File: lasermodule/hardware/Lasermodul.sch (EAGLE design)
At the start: 78 parts, among them IC1 MEGA8-AI

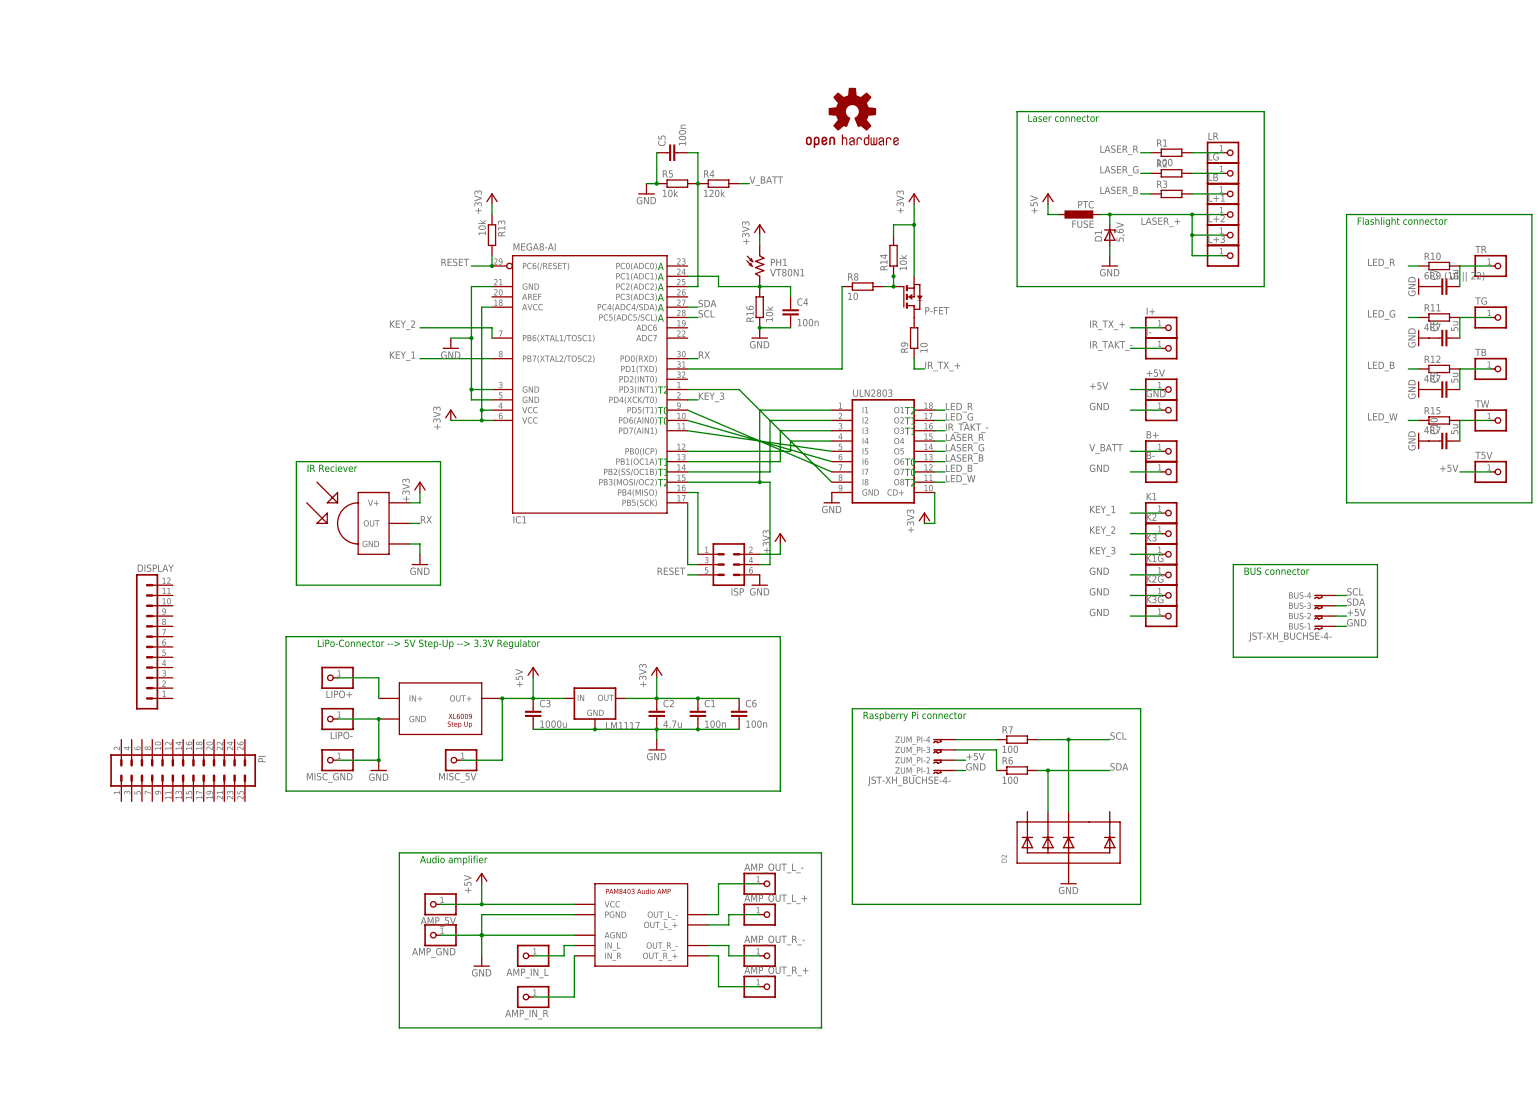
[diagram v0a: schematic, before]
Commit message: weiter gemacht
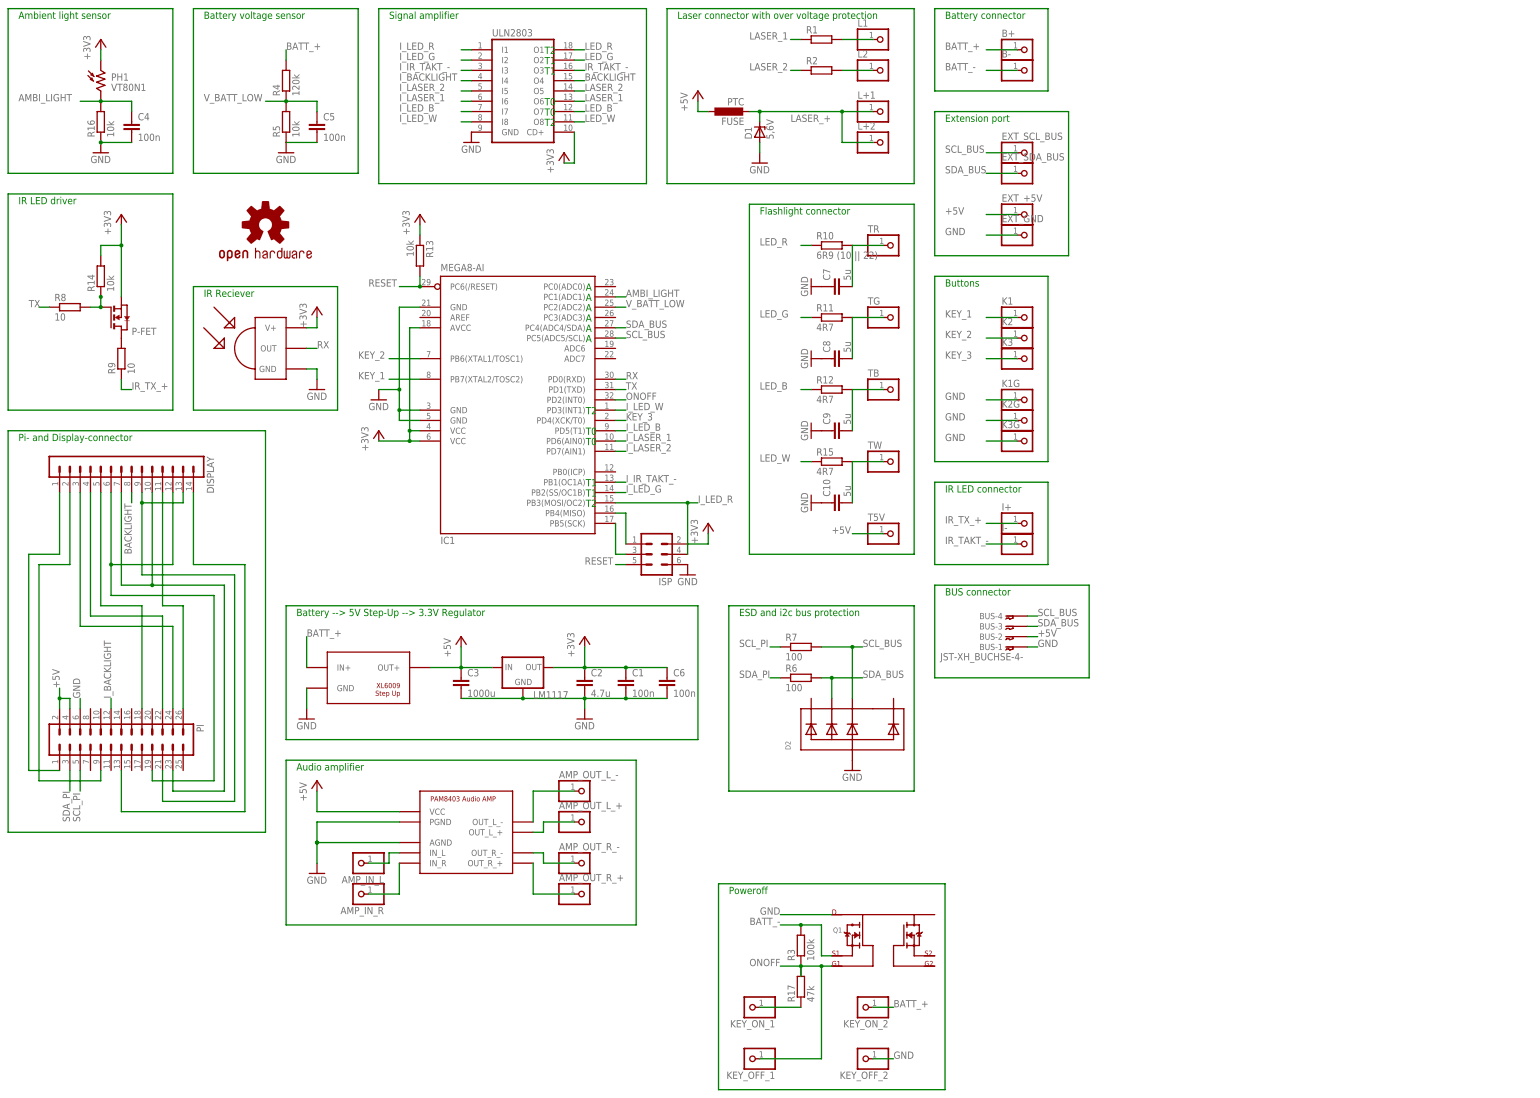
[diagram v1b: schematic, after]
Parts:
- removed +5V, AMP_5V, AMP_GND, GND, L+3, LB, LG, LIPO+, LIPO-, LR, MISC_5V, MISC_GND: (no value), wz:PIN-HEADER-1
- removed ZUM_PI: JST-XH_BUCHSE-4-, wz:JST-XH_BUCHSE-4-
- added EXT_+5V, EXT_GND, EXT_SCL_BUS, EXT_SDA_BUS, KEY_OFF_1, KEY_OFF_2, KEY_ON_1, KEY_ON_2, L1, L2: (no value), wz:PIN-HEADER-1
- added Q1: (no value), wz:CEG8205_DOPPEL_N_FET
- added R17: 47k, wz:R_EU0603
- DISPLAY: device con-lstb:MA12-1 -> wz:PIN-HEADER-DISPLAY
- R1: value 100 -> (none)
- R3: value (none) -> 100k
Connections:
- net LASER_G renamed LASER_2
- net N$1 renamed I_LED_R
- net N$10 renamed I_LED_B
- net N$17 renamed TX
- net N$2 renamed I_LED_G
- net N$26 renamed AMBI_LIGHT
- net N$3 renamed I_IR_TAKT_-
- net N$7 renamed I_LASER_2
- net N$8 renamed I_LED_W
- net N$9 renamed I_LASER_1
- removed net LASER_B: R3.1, ULN2803.O6
- removed net LASER_R: R1.1, ULN2803.O4
- removed net N$14: C5.2, IC1.PC2(ADC2), R4.1, R5.2
- removed net N$19: LB.1, R3.2
- removed net N$27: R7.1, ZUM_PI-4.1
- removed net N$28: R6.1, ZUM_PI-3.1
- removed net N$34: LIPO+.1, U$3.IN+
- removed net N$4: IC1.PB0(ICP), ULN2803.I4
- removed net SCL: BUS-4.1, D2.C3, IC1.PC5(ADC5/SCL), R7.2
- removed net SDA: BUS-3.1, D2.C2, IC1.PC4(ADC4/SDA), R6.2
- removed net V_BATT: B+.1, R4.2
- new net BACKLIGHT: DISPLAY.8, ULN2803.O4
- new net BATT_+: B+.1, KEY_ON_2.1, R4.2, U$3.IN+
- new net BATT_-: B-.1, Q1.S1, R3.2
- new net I_BACKLIGHT: PI.12, ULN2803.I4
- new net LASER_1: R1.1, ULN2803.O6
- new net N$1: DISPLAY.14, PI.13
- new net N$2: DISPLAY.11, PI.26
- new net N$26: KEY_ON_1.1, R17.1
- new net N$44: DISPLAY.1, PI.1
- new net N$45: DISPLAY.2, PI.9
- new net N$47: DISPLAY.5, PI.18
- new net N$48: DISPLAY.12, DISPLAY.6, PI.19
- new net N$49: DISPLAY.13, DISPLAY.9, PI.21
- new net N$50: DISPLAY.4, PI.22
- new net N$51: DISPLAY.10, DISPLAY.7, PI.23
- new net N$52: DISPLAY.3, PI.24
- new net ONOFF: IC1.PD2(INT0), KEY_OFF_1.1, Q1.G1, R17.2, R3.1
- new net SCL_BUS: BUS-4.1, D2.C3, EXT_SCL_BUS.1, IC1.PC5(ADC5/SCL), R7.2
- new net SCL_PI: PI.5, R7.1
- new net SDA_BUS: BUS-3.1, D2.C2, EXT_SDA_BUS.1, IC1.PC4(ADC4/SDA), R6.2
- new net SDA_PI: PI.3, R6.1
- new net V_BATT_LOW: C5.1, IC1.PC2(ADC2), R4.1, R5.2
- net +5V: now also EXT_+5V.1, PI.2, PI.4; no longer +5V.1, AMP_5V.1, MISC_5V.1, ZUM_PI-2.1
- net GND: now also C5.2, EXT_GND.1, KEY_OFF_2.1, PI.6, Q1.D; no longer AMP_GND.1, B-.1, C5.1, GND.1, LIPO-.1, MISC_GND.1, ZUM_PI-1.1
- net LASER_+: no longer L+3.1
- net N$12: now also L1.1; no longer LR.1
- net N$18: now also L2.1; no longer LG.1
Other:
- note added: "Ambient light sensor"
- note added: "Battery --> 5V Step-Up --> 3.3V Regulator"
- note added: "Battery connector"
- note added: "Battery voltage sensor"
- note added: "Buttons"
- note added: "ESD and i2c bus protection"
- note added: "Extension port"
- note added: "IR LED connector"
- note added: "IR LED driver"
- note added: "Laser connector with over voltage protection"
- note added: "Pi- and Display-connector"
- note added: "Poweroff"
- note added: "Signal amplifier"
- note removed: "Laser connector"
- note removed: "LiPo-Connector --> 5V Step-Up --> 3.3V Regulator"
- note removed: "Raspberry Pi connector"
- moved on the sheet: AMP_IN_L, AMP_IN_R, AMP_OUT_L_+, AMP_OUT_L_-, AMP_OUT_R_+, AMP_OUT_R_-, B+, B-, BUS-1, BUS-2, BUS-3, BUS-4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
